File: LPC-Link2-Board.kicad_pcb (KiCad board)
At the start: 2 copper layers, 75.2 x 49.8 mm, 9 parts, among them J2 CONN_02X05, J3 CONN_02X07, J4 CONN_02X10, J6 CONN_01X09, J7 CONN_02X05, J8 CONN_02X10, J9 CONN_02X12

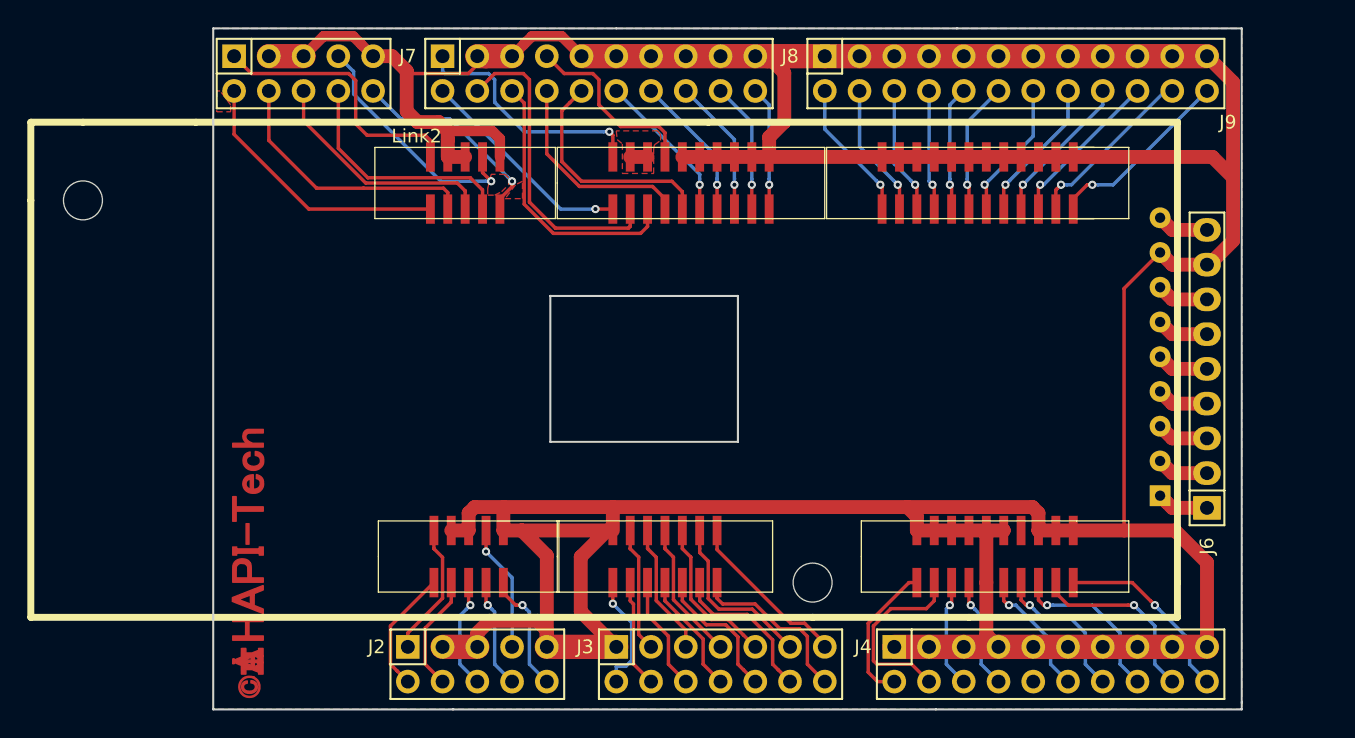
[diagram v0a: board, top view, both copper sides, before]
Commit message: no message
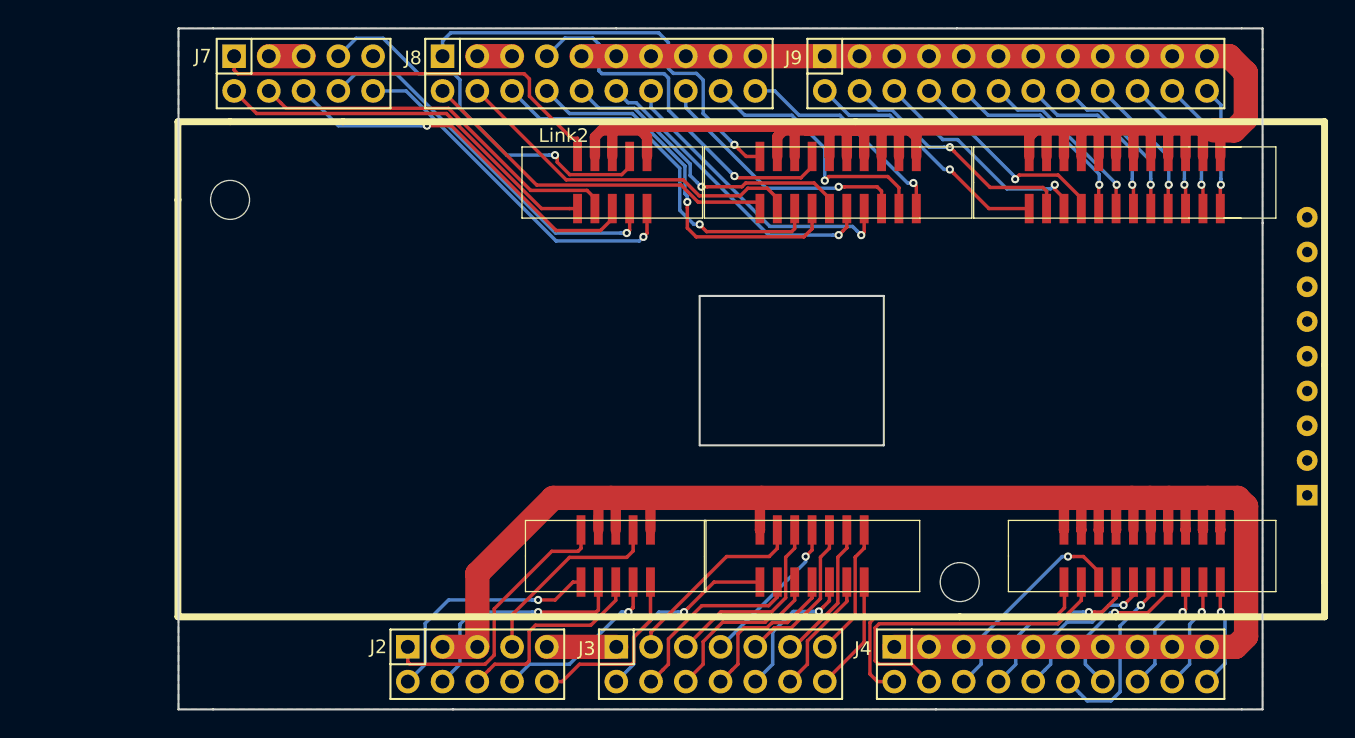
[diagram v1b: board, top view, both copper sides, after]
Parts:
- removed G***: LOGO, logo:logo_F_Cu_h2.3
- removed J6: CONN_01X09, Socket_Strips:Socket_Strip_Straight_1x09
- moved Link2 10.8 mm to (182.6, 96.6)
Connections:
- J4 pad 10: (no net) -> Net-(J4-Pad10)
- Link2 pad 4-10: GND -> Net-(J4-Pad10)
- Link2 pad 4-13: (no net) -> GND
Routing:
- net GND: track 333.4 -> 287.1 mm
- net Net-(J8-Pad7): track 13.8 -> 27.8 mm, vias 0 -> 1
- net Net-(J8-Pad1): track 18.0 -> 30.8 mm
- net Net-(J8-Pad8): track 15.3 -> 28.1 mm, vias 0 -> 1
- net Net-(J4-Pad10): track 0.00 -> 12.0 mm, vias 0 -> 1
- net Net-(J8-Pad14): track 10.6 -> 22.5 mm
- net Net-(J4-Pad2): track 10.6 -> 22.3 mm
- net Net-(J8-Pad12): track 11.2 -> 22.8 mm
- net Net-(J7-Pad10): track 15.3 -> 26.6 mm
- net Net-(J7-Pad8): track 17.4 -> 28.3 mm, vias 0 -> 1
- net Net-(J8-Pad2): track 16.0 -> 26.9 mm, vias 1 -> 0
- net Net-(J2-Pad1): track 9.82 -> 20.7 mm
- net Net-(J7-Pad6): track 17.4 -> 27.9 mm, vias 0 -> 1
- net Net-(J4-Pad4): track 13.8 -> 24.2 mm
- net Net-(J7-Pad7): track 18.0 -> 28.4 mm
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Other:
- board size 75.2 x 49.8 mm -> 79.2 x 49.8 mm
- board text added: "1 2"
- board text added: "1:JTAG-VREF 2:JTAG_TMS_SWDIO"
- board text added: "Jx"
